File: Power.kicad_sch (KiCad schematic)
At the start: 20 parts, among them IC1 LM74502HDDFR, J1 CarLVPowerConnector, J3 Conn_01x02, Q1 PSMN8R5-40MSDX

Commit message: more bom stuff
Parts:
- C21, C3: footprint Capacitor_SMD:C_0603_1608Metric -> Capacitor_SMD:C_0805_2012Metric
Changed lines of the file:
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@@
 			)
 		)
-		(property "Footprint" "Capacitor_SMD:C_0603_1608Metric"
+		(property "Footprint" "Capacitor_SMD:C_0805_2012Metric"
 			(at 112.7252 51.435 0)
 			(effects
@@
 			)
 		)
-		(property "Footprint" "Capacitor_SMD:C_0603_1608Metric"
+		(property "Footprint" "Capacitor_SMD:C_0805_2012Metric"
 			(at 204.8002 48.895 0)
 			(effects

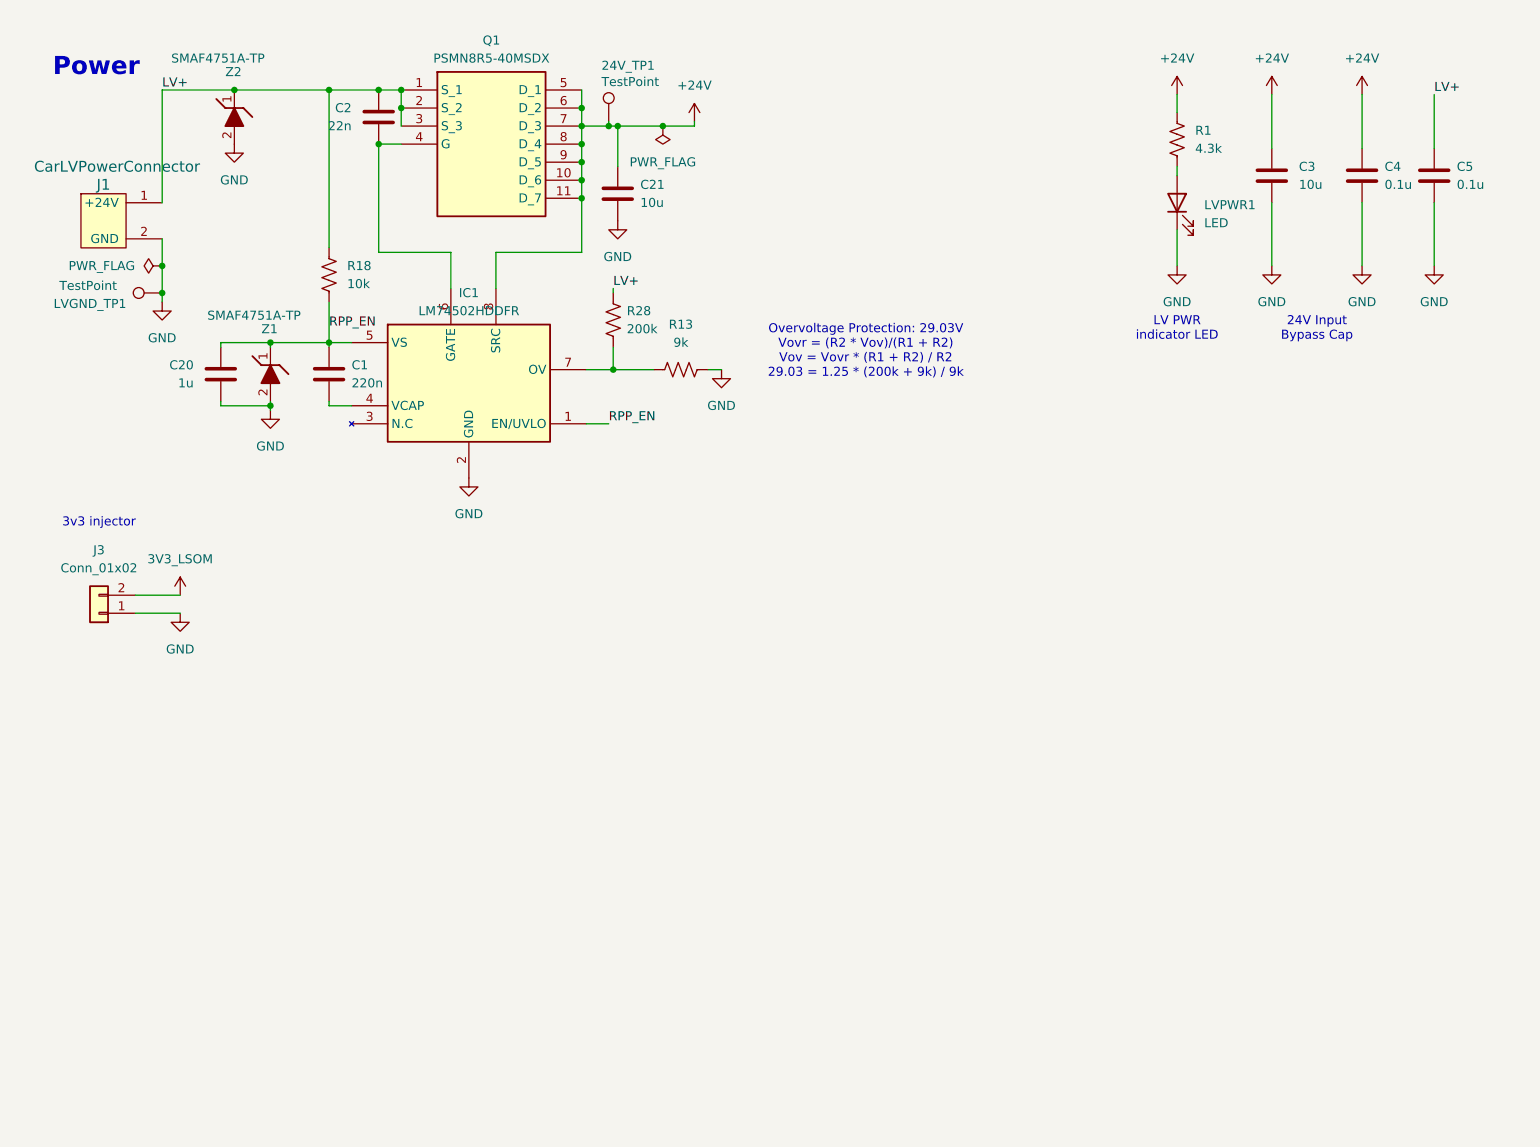
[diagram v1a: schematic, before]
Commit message: start of RevB. BOM for revA
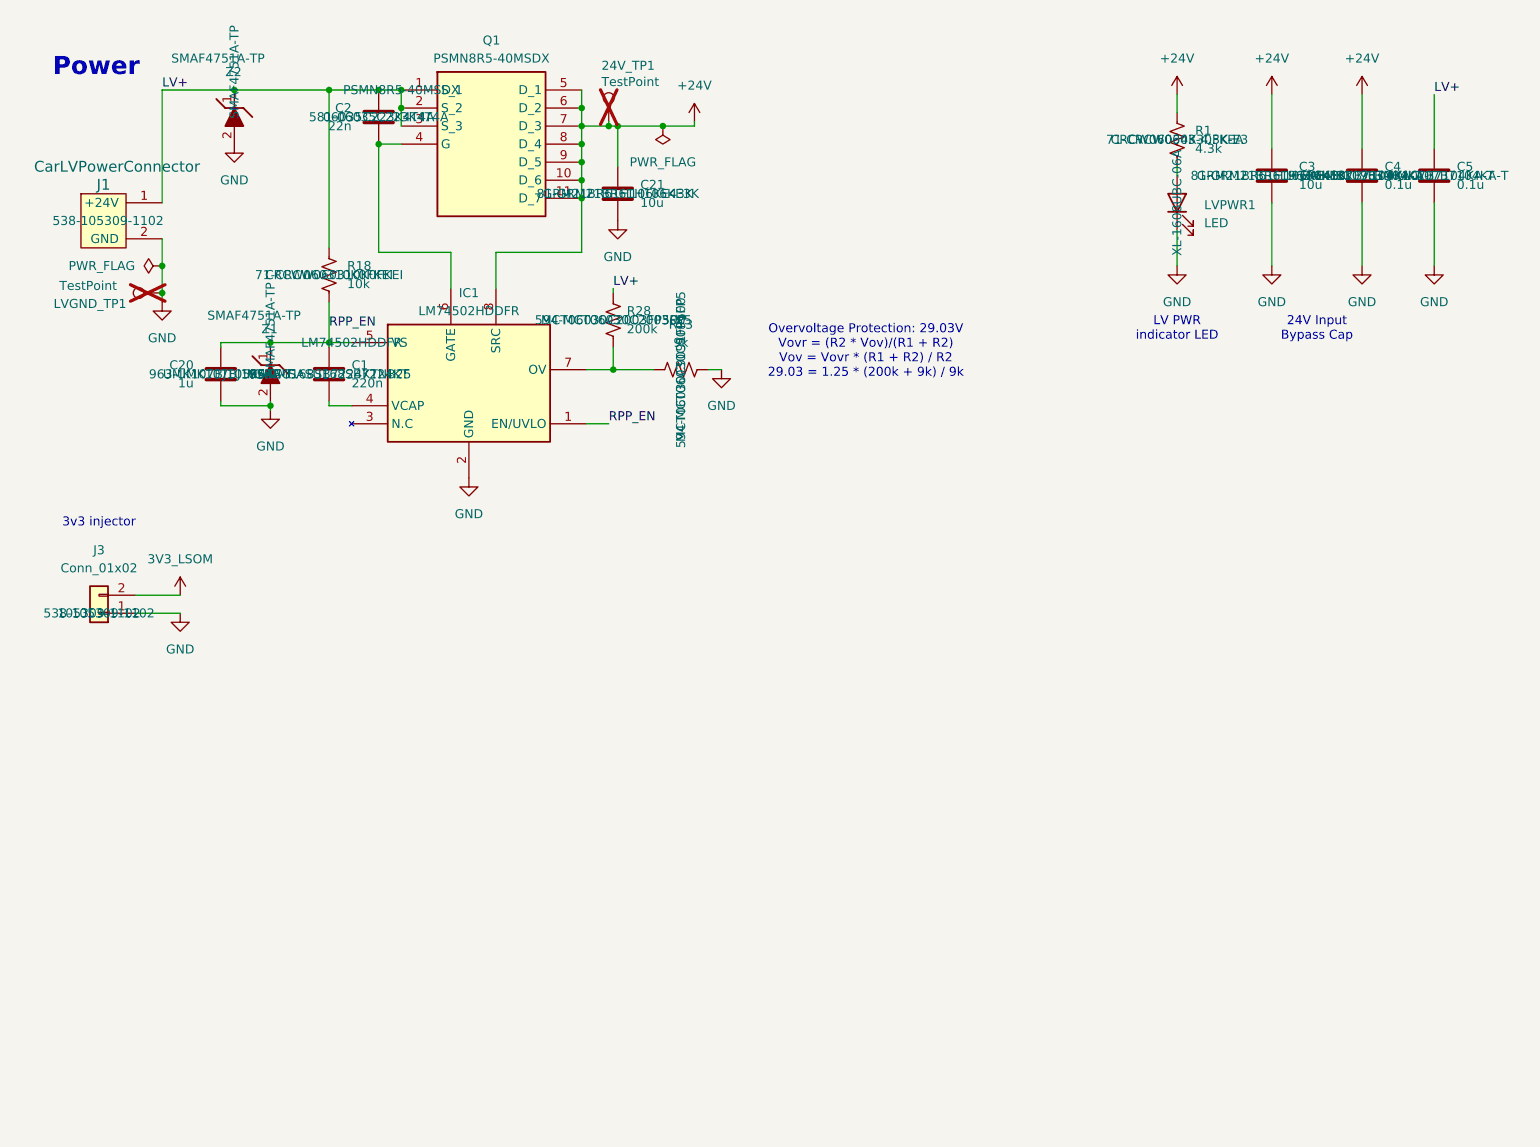
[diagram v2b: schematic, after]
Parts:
- 24V_TP1, LVGND_TP1: now not fitted; now left out of the parts list
- C1: Mouser Part Number (none) -> 963-MSASU168SB7224KT; P/N (none) -> MSASU168SB7224KTNB25
- C2: Mouser Part Number (none) -> 581-06035C223K4T4A; P/N (none) -> 06035C223K4T4A
- C20: Mouser Part Number (none) -> 963-UMK107BJ105KA-T; P/N (none) -> UMK107BJ105KA-T
- C21, C3: Mouser Part Number (none) -> 81-GRM21BR61H106KE3K; P/N (none) -> GRM21BR61H106KE43K
- C4, C5: Mouser Part Number (none) -> 963-HMK107B7104KA-T; P/N (none) -> HMK107B7104KA-T
- IC1: P/N (none) -> LM74502HDDFR
- J1, J3: Mouser Part Number (none) -> 538-105309-1102; P/N (none) -> 105309-1102
- LVPWR1: P/N (none) -> XL-1608UBC-06A
- Q1: P/N (none) -> PSMN8R5-40MSDX
- R1: Mouser Part Number (none) -> 71-CRCW0603-4.3K-E3; P/N (none) -> CRCW06034K30FKEA
- R13: Mouser Part Number (none) -> 594-MCT06030C9091FP5; P/N (none) -> MCT06030C9091FP500
- R18: Mouser Part Number (none) -> 71-CRCW060310K0FKEI; P/N (none) -> CRCW060310K0FKEI
- R28: Mouser Part Number (none) -> 594-MCT06030C2003FP5; P/N (none) -> MCT06030C2003FP500
- Z1, Z2: P/N (none) -> SMAF4751A-TP

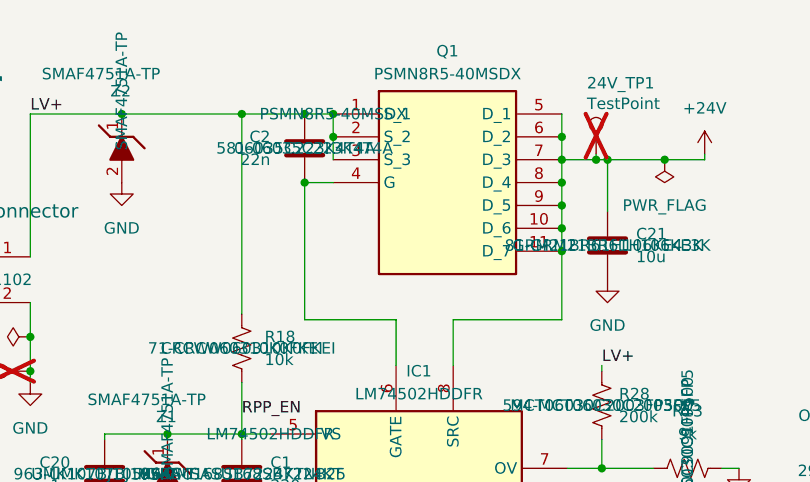
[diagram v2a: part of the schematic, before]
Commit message: changxu's symbol stuff
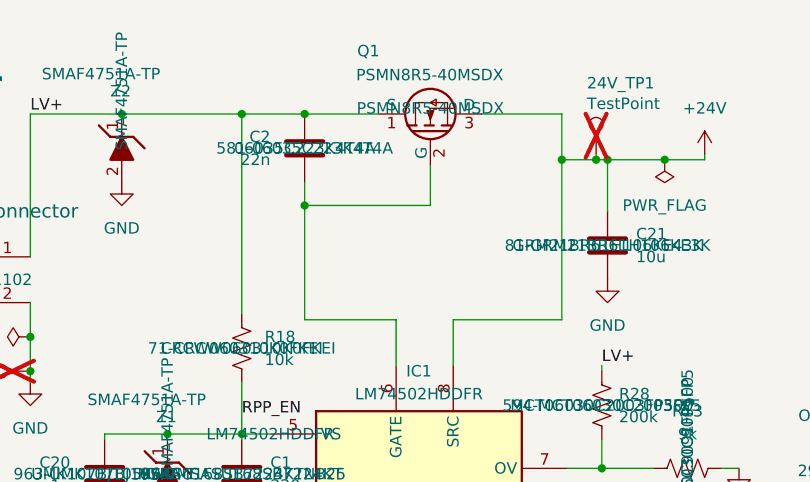
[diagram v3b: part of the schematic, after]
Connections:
- net +24V: now also Q1.3 (D); no longer Q1.10 (D_6), Q1.11 (D_7), Q1.5 (D_1), Q1.6 (D_2), Q1.7 (D_3), Q1.8 (D_4), Q1.9 (D_5)
- net LV+: no longer Q1.2 (S_2), Q1.3 (S_3)
- net at C2.1, IC1.6 (GATE): now also Q1.2 (G); no longer Q1.4 (G)
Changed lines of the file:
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@@
-	)
-	(junction
-		(at 106.68 40.64)
-		(diameter 0)
-		(color 0 0 0 0)
 	)
 	(junction
@@
 	)
 	(junction
-		(at 81.28 33.02)
-		(diameter 0)
-		(color 0 0 0 0)
-	)
-	(junction
 		(at 47.625 57.785)
 		(diameter 0)
@@
 	)
 	(junction
-		(at 106.68 43.18)
-		(diameter 0)
-		(color 0 0 0 0)
-	)
-	(junction
 		(at 57.785 33.02)
 		(diameter 0)
@@
 	)
 	(junction
-		(at 81.28 35.56)
-		(diameter 0)
-		(color 0 0 0 0)
-	)
-	(junction
 		(at 78.105 33.02)
 		(diameter 0)
@@
 	)
 	(junction
-		(at 78.105 40.64)
-		(diameter 0)
-		(color 0 0 0 0)
-	)
-	(junction
 		(at 111.76 38.1)
 		(diameter 0)
@@
 	)
 	(junction
-		(at 106.68 35.56)
-		(diameter 0)
-		(color 0 0 0 0)
-	)
-	(junction
 		(at 111.125 72.39)
 		(diameter 0)
@@
 	)
 	(junction
+		(at 78.105 43.18)
+		(diameter 0)
+		(color 0 0 0 0)
+	)
+	(junction
 		(at 62.865 68.58)
 		(diameter 0)
@@
 		(color 0 0 0 0)
 	)
-	(junction
-		(at 106.68 45.72)
-		(diameter 0)
-		(color 0 0 0 0)
-	)
-	(junction
-		(at 106.68 48.26)
-		(diameter 0)
-		(color 0 0 0 0)
-	)
 	(wire
 		(pts
@@
 	(wire
 		(pts
-			(xy 106.68 38.1) (xy 106.68 40.64)
+			(xy 106.68 38.1) (xy 106.68 55.88)
 		)
 		(stroke
@@
 	(wire
 		(pts
-			(xy 106.68 43.18) (xy 106.68 45.72)
-		)
-		(stroke
-			(width 0)
-			(type default)
-		)
-	)
-	(wire
-		(pts
 			(xy 62.865 68.58) (xy 62.865 69.215)
 		)
@@
 	(wire
 		(pts
-			(xy 106.68 40.64) (xy 106.68 43.18)
-		)
-		(stroke
-			(width 0)
-			(type default)
-		)
-	)
-	(wire
-		(pts
 			(xy 47.625 57.785) (xy 47.625 61.595)
 		)
@@
 	(wire
 		(pts
-			(xy 81.28 33.02) (xy 81.28 35.56)
+			(xy 97.79 33.02) (xy 106.68 33.02)
 		)
 		(stroke
@@
 	(wire
 		(pts
-			(xy 81.28 35.56) (xy 81.28 38.1)
+			(xy 78.105 43.18) (xy 78.105 40.64)
 		)
 		(stroke
@@
 	(wire
 		(pts
-			(xy 78.105 33.02) (xy 81.28 33.02)
-		)
-		(stroke
-			(width 0)
-			(type default)
-		)
-	)
-	(wire
-		(pts
 			(xy 106.68 38.1) (xy 110.49 38.1)
 		)
@@
 	(wire
 		(pts
-			(xy 106.68 48.26) (xy 106.68 55.88)
-		)
-		(stroke
-			(width 0)
-			(type default)
-		)
-	)
-	(wire
-		(pts
 			(xy 62.865 68.58) (xy 71.12 68.58)
 		)
@@
 	(wire
 		(pts
-			(xy 106.68 45.72) (xy 106.68 48.26)
+			(xy 92.075 38.735) (xy 92.075 43.18)
 		)
 		(stroke
@@
 	(wire
 		(pts
-			(xy 106.68 33.02) (xy 106.68 35.56)
-		)
-		(stroke
-			(width 0)
-			(type default)
-		)
-	)
-	(wire
-		(pts
 			(xy 71.12 77.47) (xy 74.295 77.47)
 		)
@@
 	(wire
 		(pts
-			(xy 78.105 40.64) (xy 81.28 40.64)
-		)
-		(stroke
-			(width 0)
-			(type default)
-		)
-	)
-	(wire
-		(pts
 			(xy 190.5 33.655) (xy 190.5 36.195)
 		)
@@
 	(wire
 		(pts
+			(xy 78.105 33.02) (xy 86.36 33.02)
+		)
+		(stroke
+			(width 0)
+			(type default)
+		)
+	)
+	(wire
+		(pts
 			(xy 71.12 55.245) (xy 71.12 33.02)
 		)
@@
 	(wire
 		(pts
+			(xy 106.68 33.02) (xy 106.68 38.1)
+		)
+		(stroke
+			(width 0)
+			(type default)
+		)
+	)
+	(wire
+		(pts
 			(xy 111.125 69.215) (xy 111.125 72.39)
 		)
@@
 	(wire
 		(pts
-			(xy 78.105 55.88) (xy 78.105 40.64)
+			(xy 78.105 55.88) (xy 78.105 43.18)
 		)
 		(stroke
@@
 	(wire
 		(pts
-			(xy 106.68 35.56) (xy 106.68 38.1)
-		)
-		(stroke
-			(width 0)
-			(type default)
-		)
-	)
-	(wire
-		(pts
 			(xy 111.76 38.1) (xy 110.49 38.1)
 		)
@@
 		(pts
 			(xy 226.695 33.655) (xy 226.695 41.275)
+		)
+		(stroke
+			(width 0)
+			(type default)
+		)
+	)
+	(wire
+		(pts
+			(xy 78.105 43.18) (xy 92.075 43.18)
 		)
 		(stroke
@@
 	(symbol
 		(lib_id "UTSVT_Power:PSMN8R5-40MSDX")
-		(at 81.28 33.02 0)
+		(at 92.075 32.385 0)
 		(unit 1)
 		(exclude_from_sim no)
@@
 		(on_board yes)
 		(dnp no)
-		(fields_autoplaced yes)
 		(property "Reference" "Q1"
-			(at 93.98 26.035 0)
-			(effects
-				(font
-					(size 1.27 1.27)
-				)
+			(at 83.947 25.273 0)
+			(effects
+				(font
+					(size 1.27 1.27)
+				)
+				(justify left top)
 			)
 		)
 		(property "Value" "PSMN8R5-40MSDX"
-			(at 93.98 28.575 0)
-			(effects
-				(font
-					(size 1.27 1.27)
-				)
+			(at 83.82 27.94 0)
+			(effects
+				(font
+					(size 1.27 1.27)
+				)
+				(justify left top)
 			)
 		)
 		(property "Footprint" "UTSVT_Power:PSMN8R5-40MSDX"
-			(at 102.87 127.94 0)
+			(at 113.665 127.305 0)
 			(effects
 				(font
@@
 		)
 		(property "Datasheet" "https://assets.nexperia.com/documents/data-sheet/PSMN8R5-40MSD.pdf"
-			(at 102.87 227.94 0)
+			(at 113.665 227.305 0)
 			(effects
 				(font
@@
 		)
 		(property "Description" "MOSFETs PSMN8R5-40MSD/SOT1210/mLFPAK"
-			(at 81.28 33.02 0)
+			(at 93.091 20.955 0)
 			(effects
 				(font
@@
 		)
 		(property "Height" "1"
-			(at 102.87 427.94 0)
+			(at 113.665 427.305 0)
 			(effects
 				(font
@@
 		)
 		(property "Mouser Part Number" "771-PSMN8R5-40MSDX"
-			(at 102.87 527.94 0)
+			(at 113.665 527.305 0)
 			(effects
 				(font
@@
 		)
 		(property "Mouser Price/Stock" "https://www.mouser.co.uk/ProductDetail/Nexperia/PSMN8R5-40MSDX?qs=vHuUswq2%252BswjdnYdBdHaPw%3D%3D"
-			(at 102.87 627.94 0)
+			(at 113.665 627.305 0)
 			(effects
 				(font
@@
 		)
 		(property "Manufacturer_Name" "Nexperia"
-			(at 102.87 727.94 0)
+			(at 113.665 727.305 0)
 			(effects
 				(font
@@
 		)
 		(property "Manufacturer_Part_Number" "PSMN8R5-40MSDX"
-			(at 102.87 827.94 0)
+			(at 113.665 827.305 0)
 			(effects
 				(font
@@
 		)
 		(property "P/N" "PSMN8R5-40MSDX"
-			(at 81.28 33.02 0)
-			(effects
-				(font
-					(size 1.27 1.27)
-				)
-			)
-		)
-		(pin "8"
-		)
-		(pin "11"
+			(at 92.075 32.385 0)
+			(effects
+				(font
+					(size 1.27 1.27)
+				)
+			)
 		)
 		(pin "1"
@@
 		(pin "3"
 		)
-		(pin "4"
-		)
-		(pin "6"
-		)
-		(pin "7"
-		)
-		(pin "5"
-		)
-		(pin "9"
-		)
-		(pin "10"
-		)
 		(instances

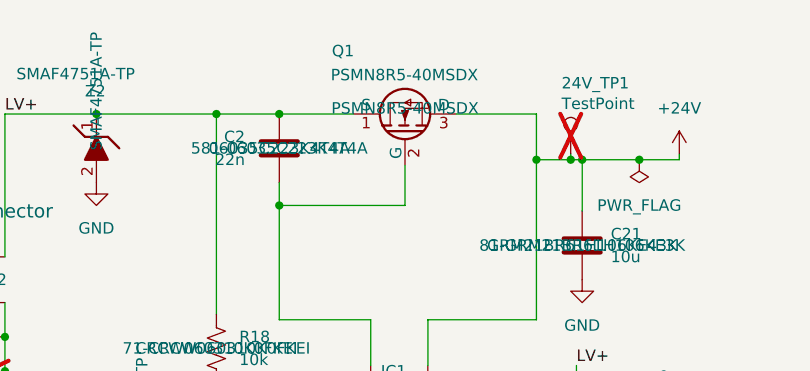
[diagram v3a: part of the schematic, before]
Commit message: rpp oopsie
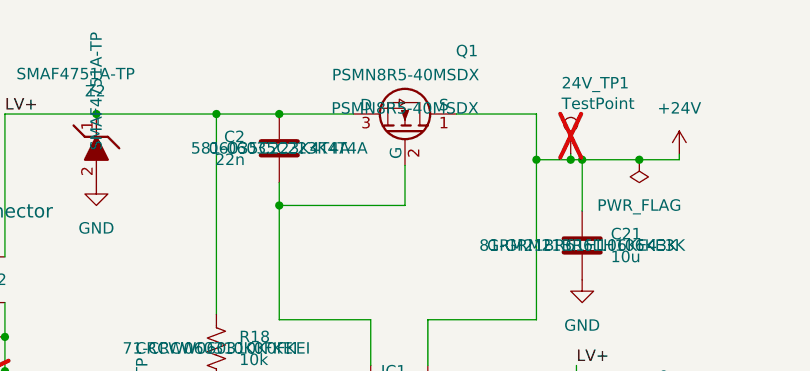
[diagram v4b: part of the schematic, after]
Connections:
- net +24V: now also Q1.1 (S); no longer Q1.3 (D)
- net LV+: now also Q1.3 (D); no longer Q1.1 (S)
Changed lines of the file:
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@@
 		(lib_id "UTSVT_Power:PSMN8R5-40MSDX")
 		(at 92.075 32.385 0)
+		(mirror y)
 		(unit 1)
 		(exclude_from_sim no)
@@
 		(dnp no)
 		(property "Reference" "Q1"
-			(at 83.947 25.273 0)
+			(at 100.203 25.273 0)
 			(effects
 				(font
@@
 		)
 		(property "Value" "PSMN8R5-40MSDX"
-			(at 83.82 27.94 0)
+			(at 100.33 27.94 0)
 			(effects
 				(font
@@
 		)
 		(property "Footprint" "UTSVT_Power:PSMN8R5-40MSDX"
-			(at 113.665 127.305 0)
+			(at 70.485 127.305 0)
 			(effects
 				(font
@@
 		)
 		(property "Datasheet" "https://assets.nexperia.com/documents/data-sheet/PSMN8R5-40MSD.pdf"
-			(at 113.665 227.305 0)
+			(at 70.485 227.305 0)
 			(effects
 				(font
@@
 		)
 		(property "Description" "MOSFETs PSMN8R5-40MSD/SOT1210/mLFPAK"
-			(at 93.091 20.955 0)
+			(at 91.059 20.955 0)
 			(effects
 				(font
@@
 		)
 		(property "Height" "1"
-			(at 113.665 427.305 0)
+			(at 70.485 427.305 0)
 			(effects
 				(font
@@
 		)
 		(property "Mouser Part Number" "771-PSMN8R5-40MSDX"
-			(at 113.665 527.305 0)
+			(at 70.485 527.305 0)
 			(effects
 				(font
@@
 		)
 		(property "Mouser Price/Stock" "https://www.mouser.co.uk/ProductDetail/Nexperia/PSMN8R5-40MSDX?qs=vHuUswq2%252BswjdnYdBdHaPw%3D%3D"
-			(at 113.665 627.305 0)
+			(at 70.485 627.305 0)
 			(effects
 				(font
@@
 		)
 		(property "Manufacturer_Name" "Nexperia"
-			(at 113.665 727.305 0)
+			(at 70.485 727.305 0)
 			(effects
 				(font
@@
 		)
 		(property "Manufacturer_Part_Number" "PSMN8R5-40MSDX"
-			(at 113.665 827.305 0)
+			(at 70.485 827.305 0)
 			(effects
 				(font

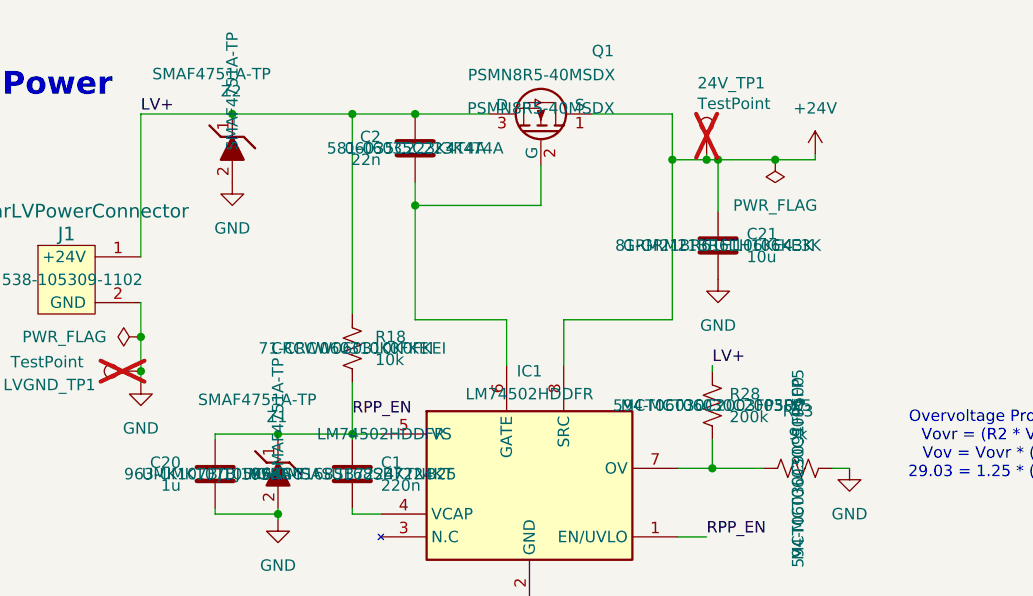
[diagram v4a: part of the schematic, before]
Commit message: kms rpp
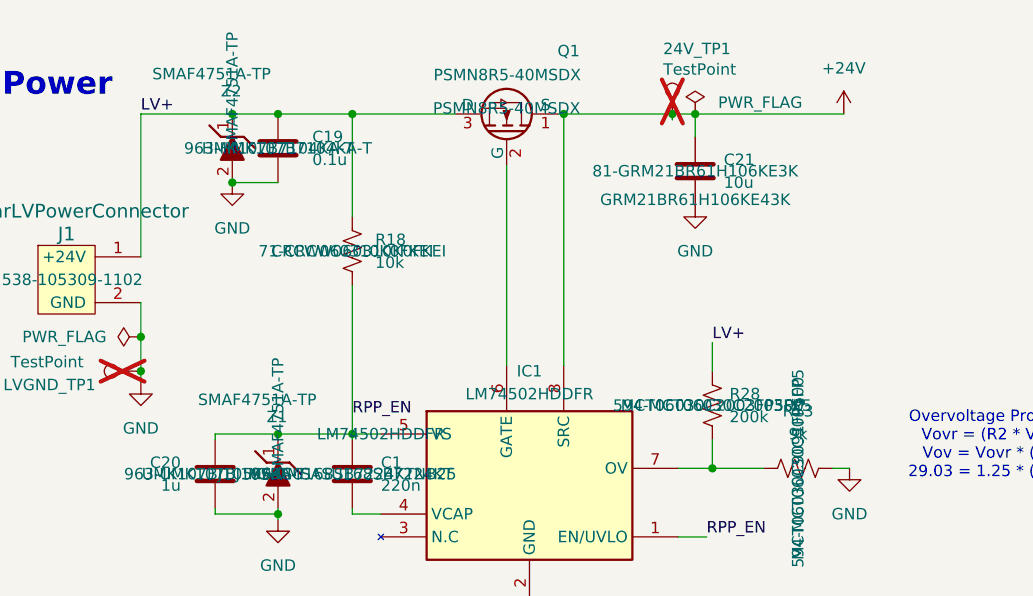
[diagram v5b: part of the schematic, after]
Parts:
- removed C2: 22n, Capacitor_SMD:C_0603_1608Metric, symbol Device:C
- added C19: 0.1u, Capacitor_SMD:C_0603_1608Metric, symbol Device:C
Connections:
- net GND: now also C19.2
- net LV+: now also C19.1
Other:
- moved on the sheet: 24V_TP1, C21, Q1, R18
